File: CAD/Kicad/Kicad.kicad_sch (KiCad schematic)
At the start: 7 parts, among them J1 USB_B_Mini, U1 AMS1117, U2 ESP8266EX

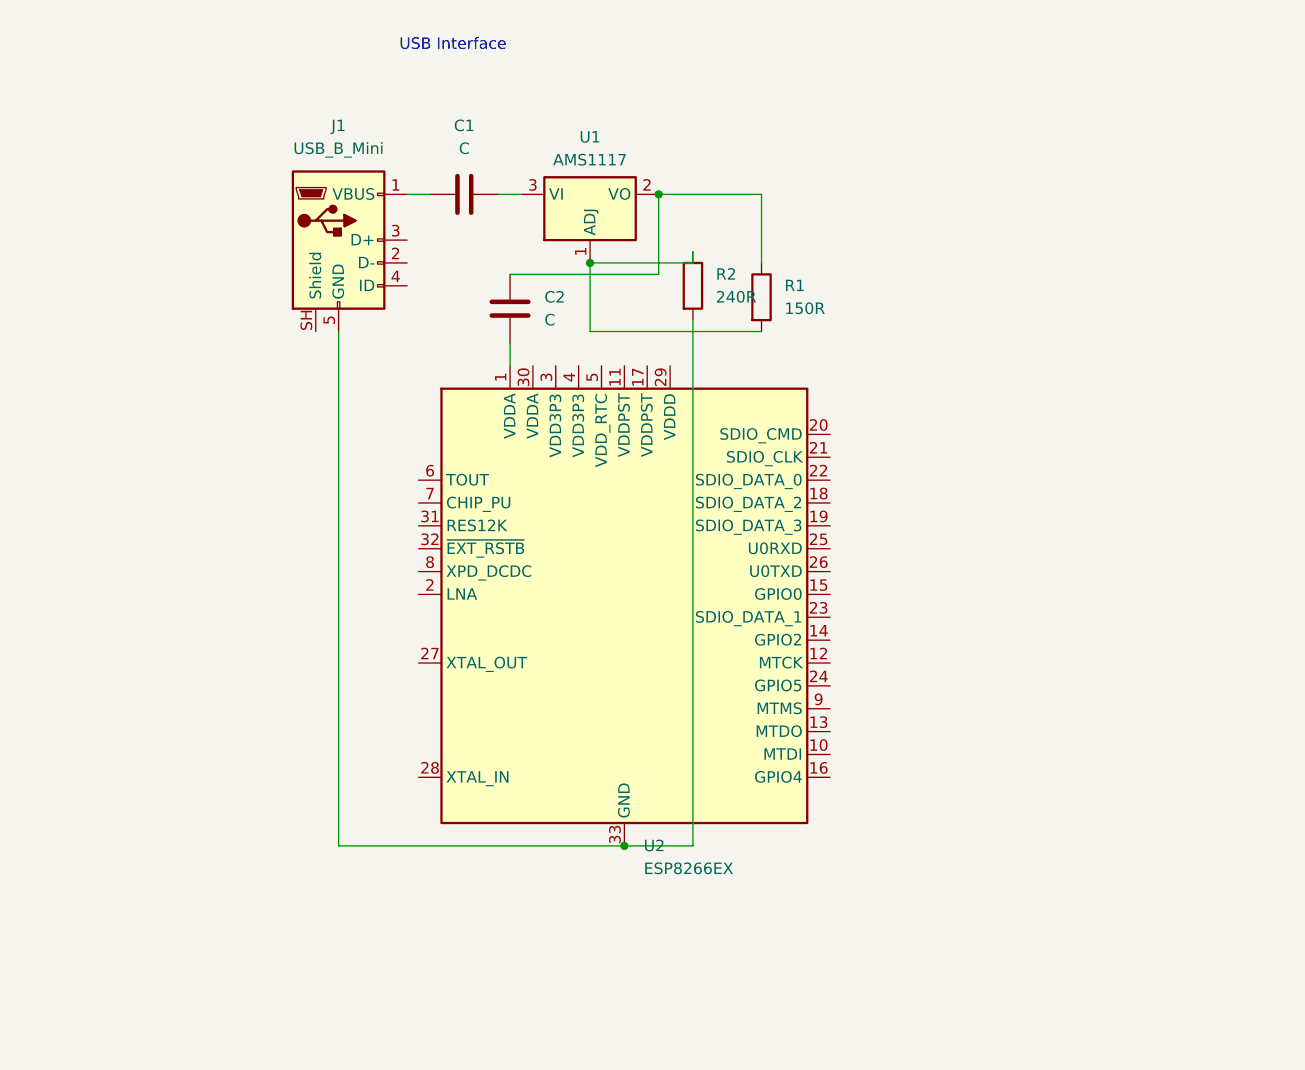
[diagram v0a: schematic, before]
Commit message: More PCB stuff
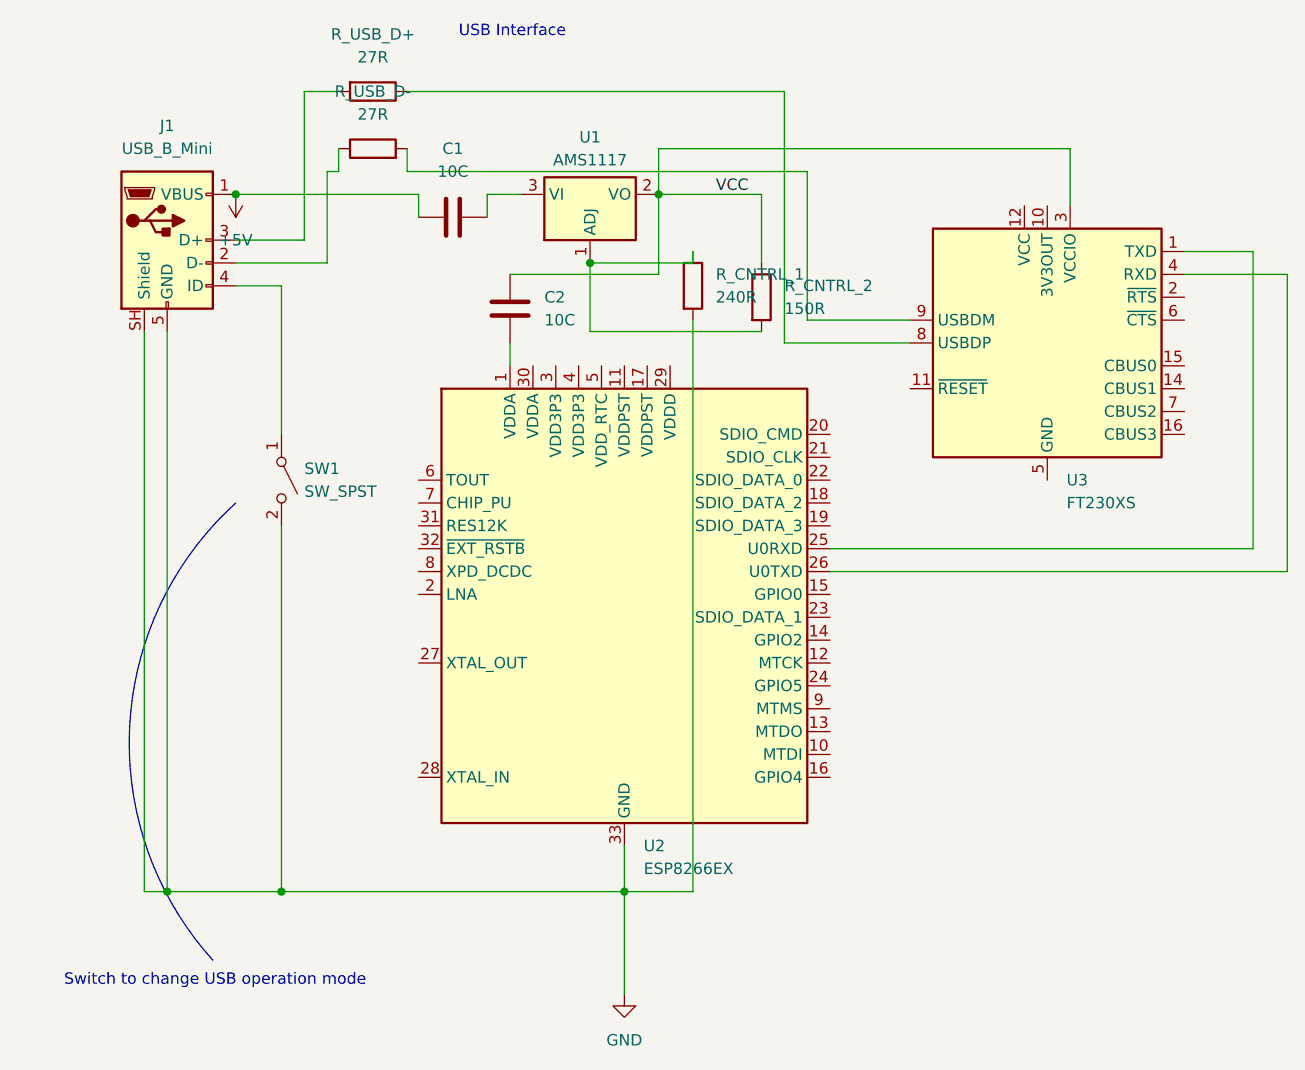
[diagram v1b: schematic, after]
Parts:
- added R_USB_D+, R_USB_D-: 27R, symbol Device:R
- added SW1: SW_SPST, symbol Switch:SW_SPST
- added U3: FT230XS, Package_SO:SSOP-16_3.9x4.9mm_P0.635mm, symbol Interface_USB:FT230XS
- C1, C2: value C -> 10C
- renumbered R2 to R_CNTRL_1, R1 to R_CNTRL_2
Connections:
- net at U2.25 (U0RXD): now also U3.1 (TXD)
- net at U2.26 (U0TXD): now also U3.4 (RXD)
- net GND: now reaches J1.5 (GND), R_CNTRL_1.2, U2.33 (GND)
- net GND: now also J1.SH (Shield), SW1.2 (B)
- net VCC: now reaches C2.1, R_CNTRL_2.1, U1.2 (VO)
- net VCC: now also U3.3 (VCCIO)
- net +5V: now reaches C1.2, J1.1 (VBUS)
- net at J1.2 (D-): now also R_USB_D-.1
- net at J1.3 (D+): now also R_USB_D+.2
- net at J1.4 (ID): now also SW1.1 (A)
- new net: R_USB_D-.2, U3.9 (USBDM)
- new net: U3.13 (GND), U3.5 (GND)
- new net: R_USB_D+.1, U3.8 (USBDP)
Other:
- note added: "Switch to change USB operation mode"
- moved on the sheet: C1, J1
